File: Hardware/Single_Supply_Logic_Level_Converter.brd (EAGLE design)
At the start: 25.4 x 25.4 mm, 23 parts, among them U1 TXB0104, U2 TPS61200, U4 MIC5219-3.3

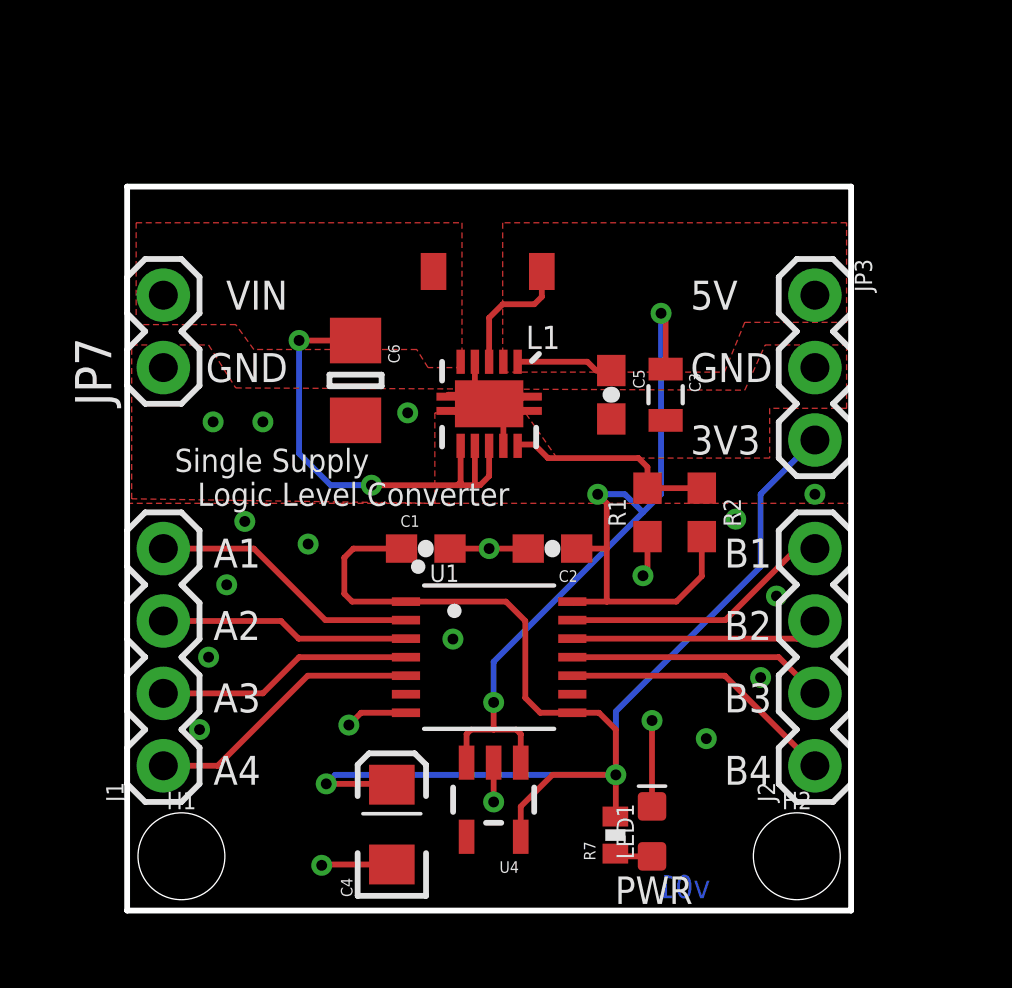
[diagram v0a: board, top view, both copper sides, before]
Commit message: Updating design per review
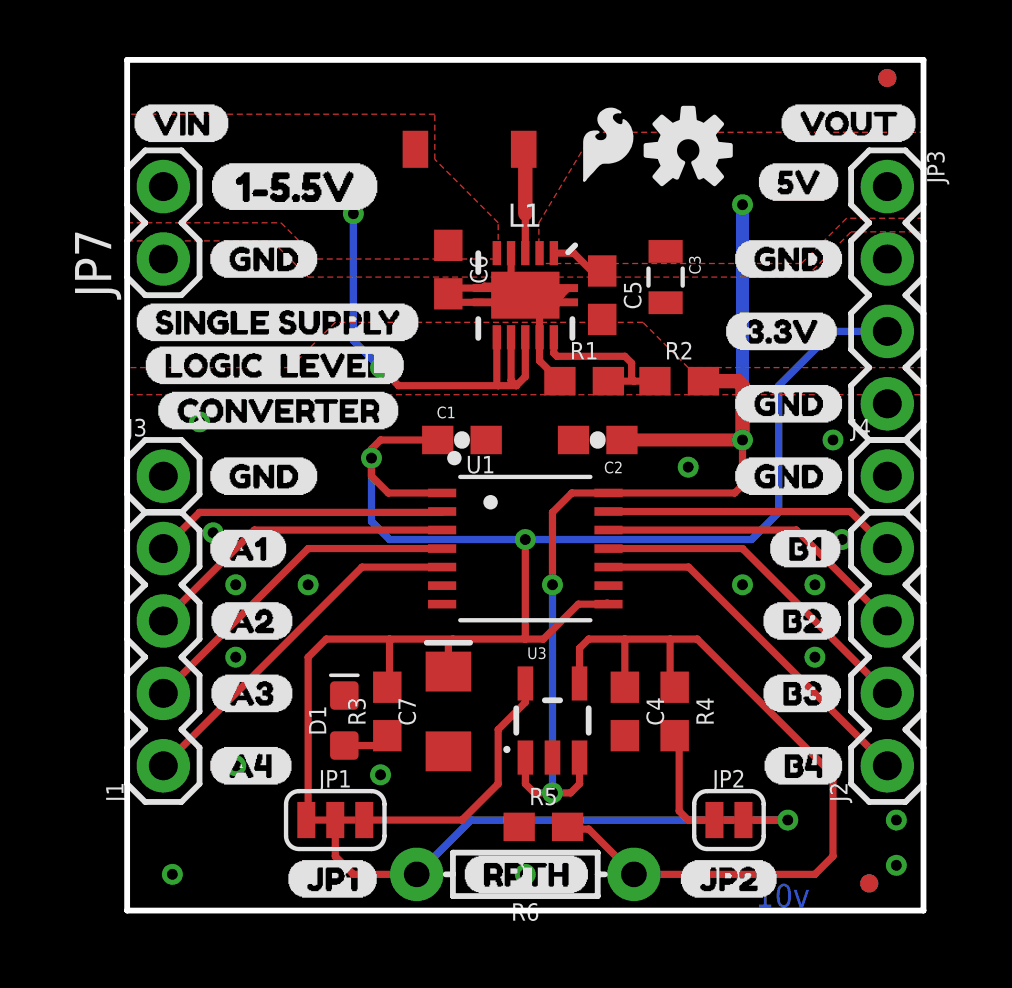
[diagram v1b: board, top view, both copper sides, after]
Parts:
- removed H1, H2: STAND-OFFTIGHT, SparkFun-Hardware:STAND-OFF-TIGHT
- removed LED1: RED, SparkFun-LED:LED-0603
- removed R7: 1K, SparkFun:0402-RES
- removed U4: MIC5219-3.3, SparkFun:SOT23-5
- added C7: 10uF, SparkFun-Capacitors:EIA3216
- added D1: RED, SparkFun-LED:LED-0603
- added FD1, FD2, FD3, FD4: FIDUCIALUFIDUCIAL, SparkFun-Aesthetics:FIDUCIAL-MICRO
- added J3, J4: (no value), SparkFun-Connectors:1X01
- added JP1: JUMPER-SMT_3_1-NC_TRACE_SILK, SparkFun-Jumpers:SMT-JUMPER_3_1-NC_TRACE_SILK
- added JP2: JUMPER-SMT_2_NC_TRACE_SILK, SparkFun-Jumpers:SMT-JUMPER_2_NC_TRACE_SILK
- added LOGO3: SFE_LOGO_FLAME.1_INCH, SparkFun-Aesthetics:SFE_LOGO_FLAME_.1
- added LOGO4: OSHW-LOGOS, SparkFun-Aesthetics:OSHW-LOGO-S
- added R3: 1k, SparkFun-Resistors:0603
- added R4: 13k, SparkFun-Resistors:0603
- added R5: 22k, SparkFun-Resistors:0603
- added R6: (no value), SparkFun-Resistors:AXIAL-0.3
- added U$10, U$38: (no value), Single_Supply_Logic_Level_Converter_Lables:A16
- added U$11, U$39: (no value), Single_Supply_Logic_Level_Converter_Lables:A27
- added U$12, U$40: (no value), Single_Supply_Logic_Level_Converter_Lables:A38
- added U$13, U$41: (no value), Single_Supply_Logic_Level_Converter_Lables:A49
- added U$14, U$46: (no value), Single_Supply_Logic_Level_Converter_Lables:B110
- added U$15, U$45: (no value), Single_Supply_Logic_Level_Converter_Lables:B211
- added U$16, U$43: (no value), Single_Supply_Logic_Level_Converter_Lables:B312
- added U$17, U$42: (no value), Single_Supply_Logic_Level_Converter_Lables:B413
- added U$18, U$36: (no value), Single_Supply_Logic_Level_Converter_Lables:CONVERTER19
- added U$19, U$26, U$30, U$31, U$32, U$33, U$37, U$47, U$48, U$50: (no value), Single_Supply_Logic_Level_Converter_Lables:GND0
- added U$20: (no value), Single_Supply_Logic_Level_Converter_Lables:JP114
- added U$21: (no value), Single_Supply_Logic_Level_Converter_Lables:JP215
- added U$22, U$35: (no value), Single_Supply_Logic_Level_Converter_Lables:LOGIC__LEVEL18
- added U$23, U$44: (no value), Single_Supply_Logic_Level_Converter_Lables:RPTH16
- added U$24, U$53: (no value), Single_Supply_Logic_Level_Converter_Lables:SINGLE_SUPPLY17
- added U$25, U$29: (no value), voltageIn:1#5#5V0
- added U$27, U$8: (no value), Single_Supply_Logic_Level_Converter_Lables:VIN1
- added U$28, U$52: (no value), Single_Supply_Logic_Level_Converter_Lables:VOUT2
- added U$49, U$7: (no value), Single_Supply_Logic_Level_Converter_Lables:3#3V20
- added U$51, U$9: (no value), Single_Supply_Logic_Level_Converter_Lables:5V3
- added U3: ADJ, SparkFun-IC-Power:SOT23-5
- C4: value 10uF -> 470pF; device SparkFun:EIA3216 -> SparkFun-Capacitors:0603
- C5: device SparkFun:0603-CAP -> SparkFun-Capacitors:0603
- C6: device CH_passive:1206 -> SparkFun-Capacitors:0603
- JP3: device SparkFun-Connectors:1X03 -> SparkFun-Connectors:1X04
- U2: device SparkFun:QFN-10_PAD -> SparkFun-IC-Power:QFN-10_PAD
- moved C4 9.09 mm to (17.5, 6.99), turned to 270 degrees
- moved R1 5.11 mm to (16.0, 18.6), turned to 0 degrees
- moved C6 5.07 mm to (11.3, 22.5)
- moved R2 4.67 mm to (19.4, 18.6), turned to 0 degrees
- moved JP3 4.58 mm to (26.7, 25.4)
- moved L1 4.33 mm to (12.0, 26.7)
- moved C2 4.13 mm to (16.5, 16.5)
- moved C3 4.13 mm to (18.9, 22.2)
- moved C1 4.02 mm to (11.7, 16.5)
- moved U1 4.02 mm to (14.0, 12.7)
- moved U2 4.02 mm to (14.0, 21.6)
- moved JP7 3.81 mm to (1.27, 22.9)
- moved C5 3.51 mm to (16.7, 21.6)
- moved J2 2.54 mm to (26.7, 5.08)
- moved FRAME1 2.25 mm to (-4.95, -10.2)
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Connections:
- removed net 3.3V: C1.1, C4.A, JP3.3, R7.2, U1.1, U1.8, U4.5
- removed net N$4: LED1.A, R7.1
- new net N$1: JP1.3, U3.5
- new net N$11: C4.1, R4.1, R5.2, R6.P$1, U3.4
- new net N$12: JP2.1, R4.2
- new net N$3: D1.A, R3.1
- new net VCCA: C1.1, C7.+, JP1.1, JP1.2, JP2.2, JP3.3, R3.2, R6.P$2, U1.1, U1.8
- net 5V: now also U3.1, U3.3; no longer U4.1, U4.3
- net GND: now also C4.2, C7.-, D1.C, J3.1, J4.1, JP3.4, R5.1, U3.2; no longer C4.C, LED1.C, U4.2
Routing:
- net VCCA: track 0.00 -> 76.6 mm, vias 0 -> 3
- net 3.3V: track 51.6 -> 0.00 mm, vias 2 -> 0
- net N$11: track 0.00 -> 28.8 mm
- net N$1: track 0.00 -> 9.14 mm
- net GND: track 19.4 -> 11.8 mm, vias 18 -> 17
- net N$12: track 0.00 -> 4.08 mm
- net B4: track 9.82 -> 12.7 mm
- net B3: track 9.04 -> 11.9 mm
- net A4: track 9.82 -> 12.7 mm
- net A3: track 9.04 -> 11.9 mm
- net B2: track 8.77 -> 11.1 mm
- net A2: track 8.77 -> 11.1 mm
- net 5V: track 36.3 -> 38.3 mm, vias 3 -> 4
- net FB: track 7.55 -> 5.89 mm
- net N$3: track 0.00 -> 1.65 mm
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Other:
- board size 25.4 x 25.4 mm -> 27.9 x 29.8 mm
- board text added: "All Units in Inches"
- board text added: "Mary West"
- board text removed: "3V3"
- board text removed: "5V"
- board text removed: "A1"
- board text removed: "A2"
- board text removed: "A3"
- board text removed: "A4"
- board text removed: "B1"
- board text removed: "B2"
- board text removed: "B3"
- board text removed: "B4"
- board text removed: "GND"
- board text removed: "Logic Level Converter"
- board text removed: "PWR"
- board text removed: "Single Supply"
- board text removed: "Single Supply Logic Level Converter"
- board text removed: "VCCA: 3.3V"
- board text removed: "VIN"
- board text removed: "VOUT"
